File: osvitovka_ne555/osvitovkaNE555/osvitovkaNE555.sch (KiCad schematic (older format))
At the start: 41 parts, among them J1 +12V, J10 Screw_Terminal_01x01, J11 Screw_Terminal_01x01, J12 Screw_Terminal_01x01, J13 Screw_Terminal_01x01, J14 Screw_Terminal_01x01, J15 Screw_Terminal_01x01, J16 Screw_Terminal_01x01, J17 Screw_Terminal_01x01, J18 Screw_Terminal_01x01, J19 Screw_Terminal_01x01, J2 gnd, J20 Screw_Terminal_01x01, J21 Screw_Terminal_01x01, J22 Screw_Terminal_01x01, J23 Screw_Terminal_01x01, J24 Screw_Terminal_01x01, J25 Screw_Terminal_01x01, J26 Screw_Terminal_01x01, J27 Screw_Terminal_01x01, J28 Screw_Terminal_01x01, J3 Screw_Terminal_01x01, J4 Screw_Terminal_01x01, J5 Screw_Terminal_01x01, J6 Screw_Terminal_01x01, J7 Screw_Terminal_01x01, J8 Screw_Terminal_01x01, J9 Screw_Terminal_01x01, K1 RSM822, Q1 BC337, SW1 Start, U1 LMC555xN

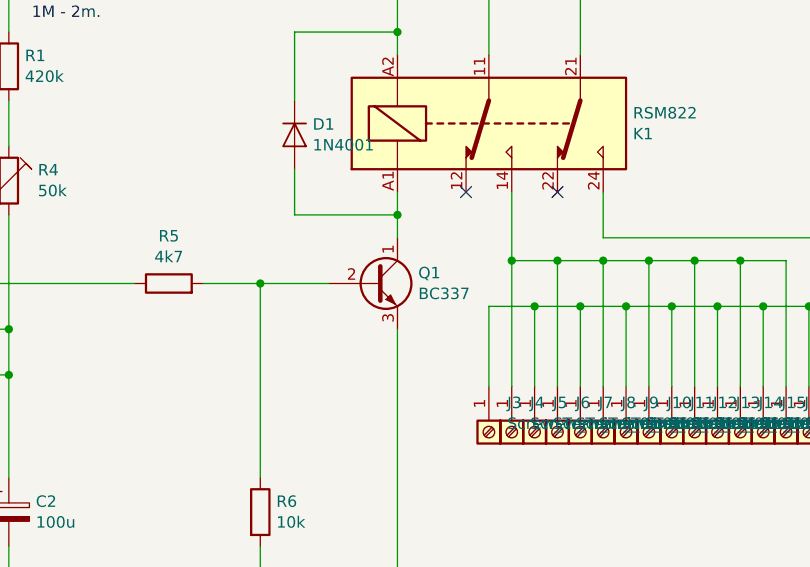
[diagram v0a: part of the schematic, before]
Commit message: test a upgrade pcb.
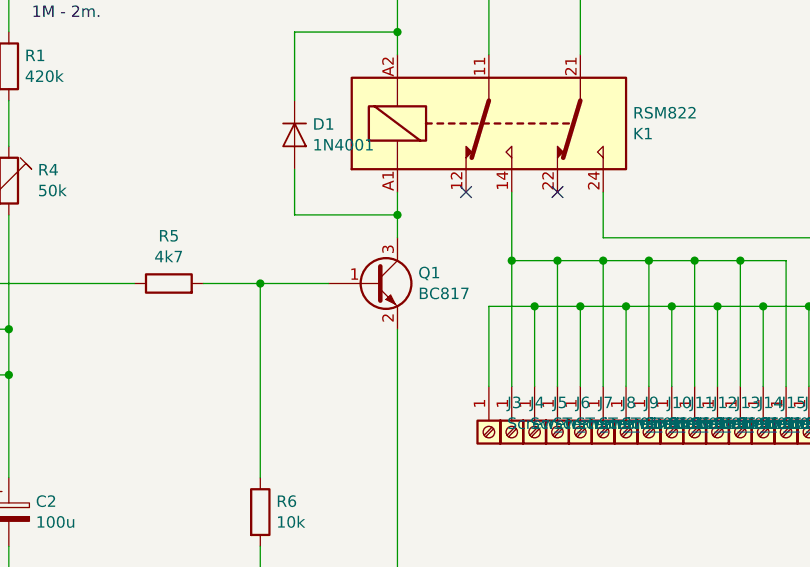
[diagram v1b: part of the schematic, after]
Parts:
- removed Q1: BC337, Package_TO_SOT_SMD:SOT-23, symbol Transistor_BJT:BC337
- added Q1: BC817, Package_TO_SOT_SMD:SOT-23, symbol Transistor_BJT:BC817
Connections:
- net GND: now also Q1.2 (E)
- net at R5.2, R6.1: now also Q1.1 (B)
- net at D1.2 (A), K1.A1: now also Q1.3 (C)
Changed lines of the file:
@@
-$EndComp
-$Comp
-L Transistor_BJT:BC337 Q1
-U 1 1 5FCFC78D
-P 7200 3350
-F 0 "Q1" H 7391 3396 50  0000 L CNN
-F 1 "BC337" H 7391 3305 50  0000 L CNN
-F 2 "Package_TO_SOT_SMD:SOT-23" H 7400 3275 50  0001 L CIN
-F 3 "https://diotec.com/tl_files/diotec/files/pdf/datasheets/bc337.pdf" H 7200 3350 50  0001 L CNN
-	1    7200 3350
-	1    0    0    -1
 $EndComp
 $Comp
@@
 Wire Wire Line
 	3050 4750 4350 4750
+$Comp
+L Transistor_BJT:BC817 Q1
+U 1 1 5FDE9E5B
+P 7200 3350
+F 0 "Q1" H 7391 3396 50  0000 L CNN
+F 1 "BC817" H 7391 3305 50  0000 L CNN
+F 2 "Package_TO_SOT_SMD:SOT-23" H 7400 3275 50  0001 L CIN
+F 3 "http://www.fairchildsemi.com/ds/BC/BC817.pdf" H 7200 3350 50  0001 L CNN
+	1    7200 3350
+	1    0    0    -1
+$EndComp
 $EndSCHEMATC
